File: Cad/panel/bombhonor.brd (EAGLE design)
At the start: 160 x 200.4 mm, 492 parts, among them U1 STM32L011F4P6, U2 STM32L011F4P6, U3 STM32L011F4P6, U4 STM32L011F4P6, U5 STM32L011F4P6, U6 STM32L011F4P6

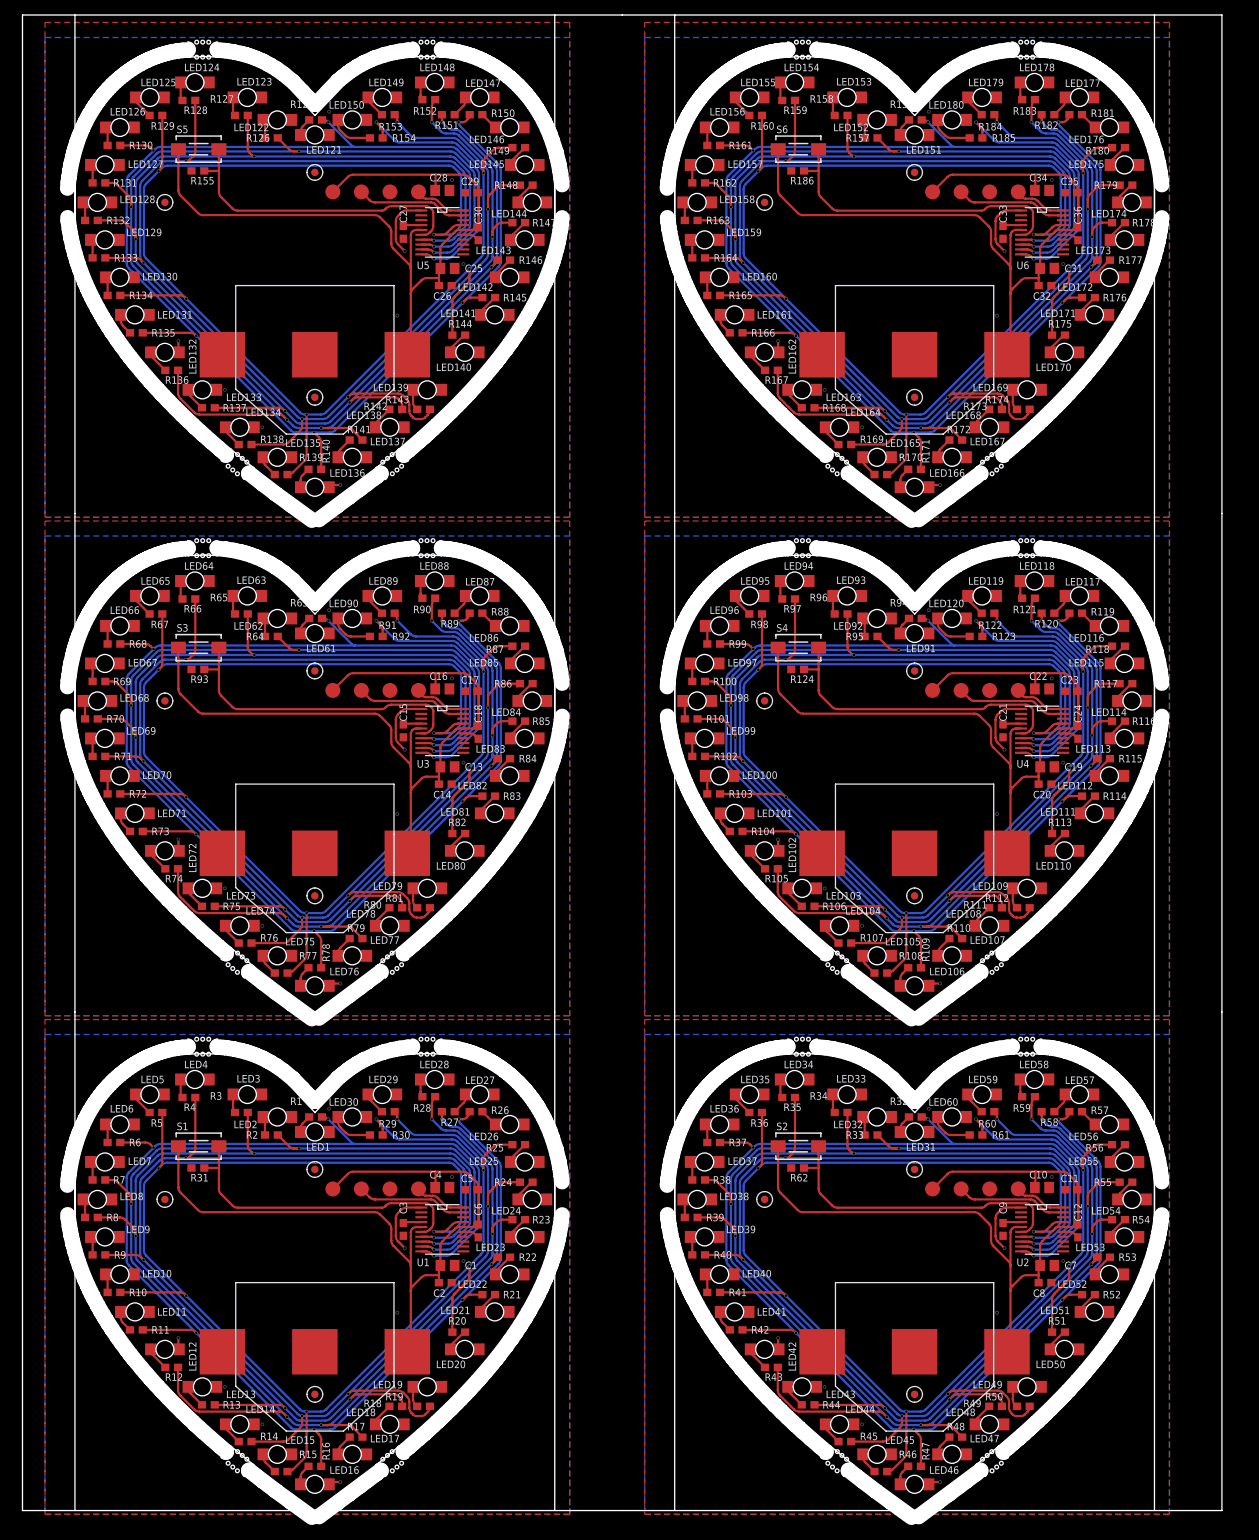
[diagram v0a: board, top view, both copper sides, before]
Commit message: messo a posto pannello
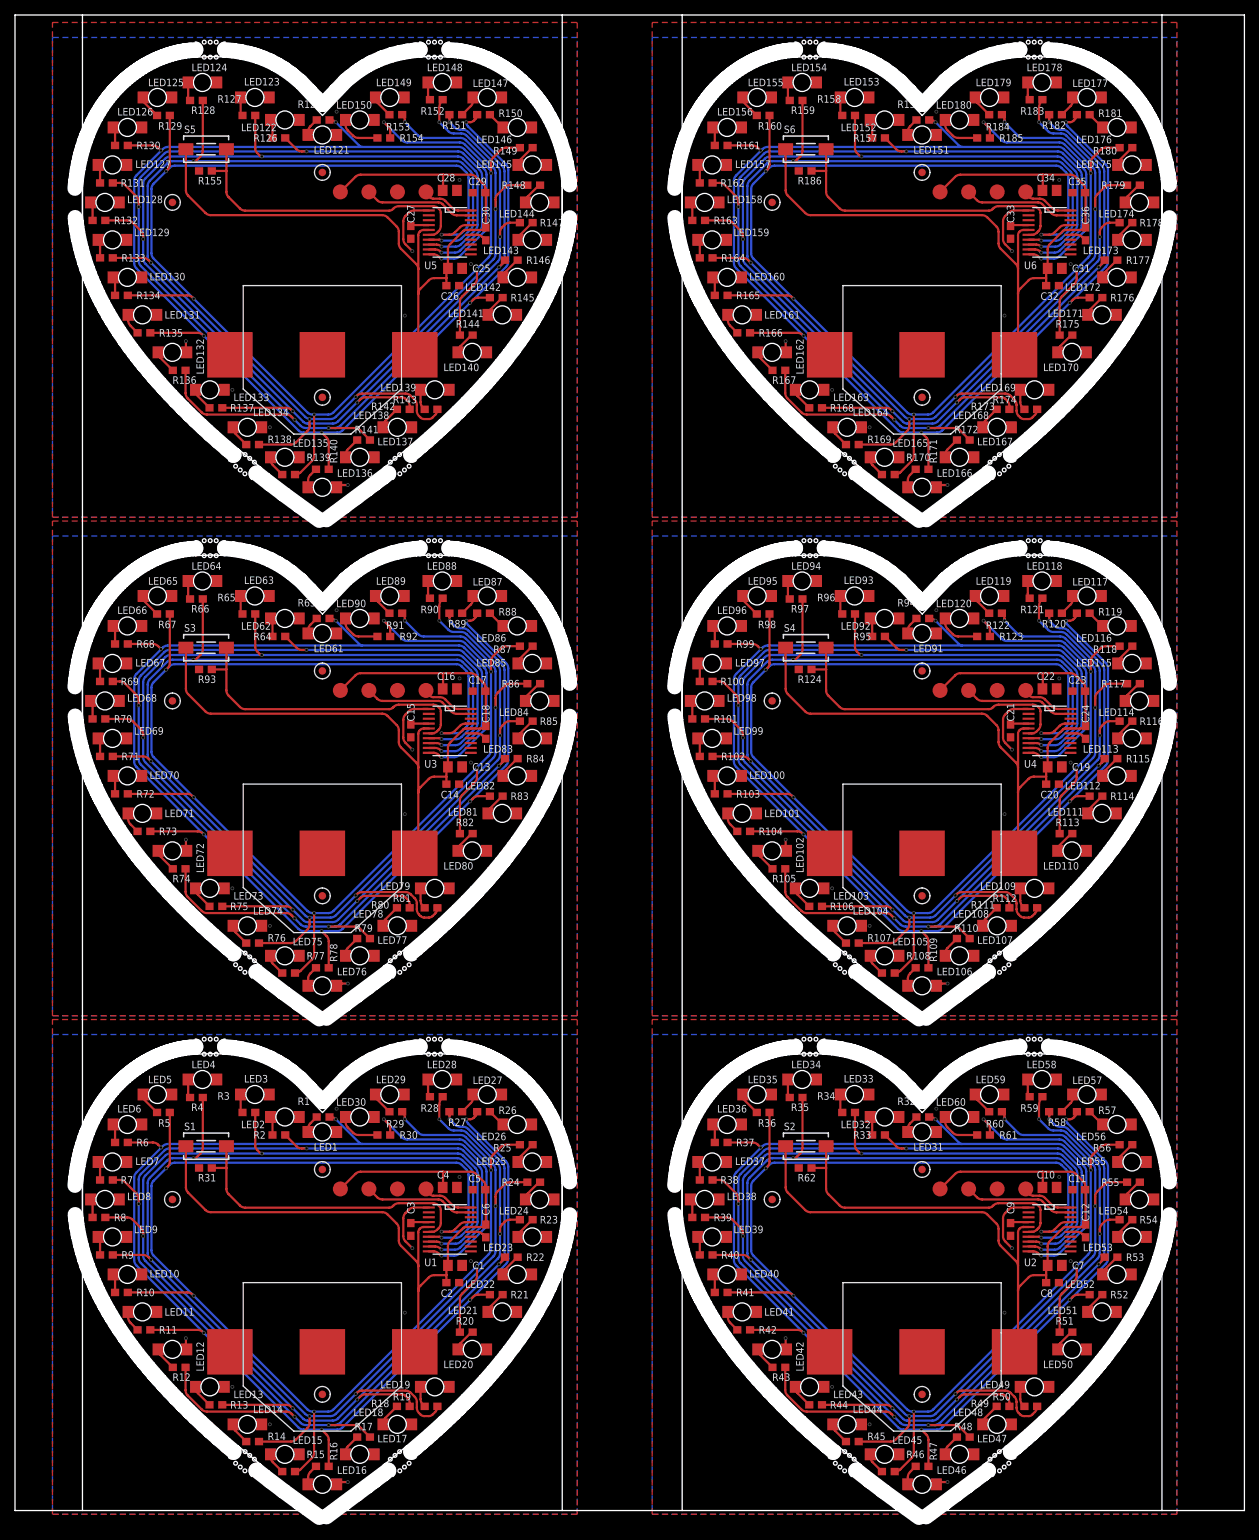
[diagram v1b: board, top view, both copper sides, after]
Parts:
- moved 1 1.00 mm to (26.0, 61.9)
- moved 10 1.00 mm to (56.0, 194.9)
- moved 11 1.00 mm to (106.0, 194.9)
- moved 12 1.00 mm to (136.0, 194.9)
- moved 2 1.00 mm to (56.0, 61.9)
- moved 3 1.00 mm to (106.0, 61.9)
- moved 4 1.00 mm to (136.0, 61.9)
- moved 5 1.00 mm to (26.0, 128.4)
- moved 6 1.00 mm to (56.0, 128.4)
- moved 7 1.00 mm to (106.0, 128.4)
- moved 8 1.00 mm to (136.0, 128.4)
- moved 9 1.00 mm to (26.0, 194.9)
- moved BATT1 1.00 mm to (41.0, 20.5)
- moved BATT2 1.00 mm to (121.0, 20.5)
- moved BATT3 1.00 mm to (41.0, 87.0)
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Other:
- board size 160 x 200.4 mm -> 164 x 200.4 mm
